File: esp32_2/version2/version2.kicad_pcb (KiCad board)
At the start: 4 copper layers, 31 x 38.5 mm, 29 parts, among them J1 USB_C_Receptacle_USB2.0_16P, J2 Conn_01x08_Pin, J3 Conn_01x08_Pin, SW1 SW_Push, SW2 SW_Push, U1 USBLC6-2SC6, U2 AP2112K-3.3, U3 ESP32-C3-WROOM-02, Y1 Crystal

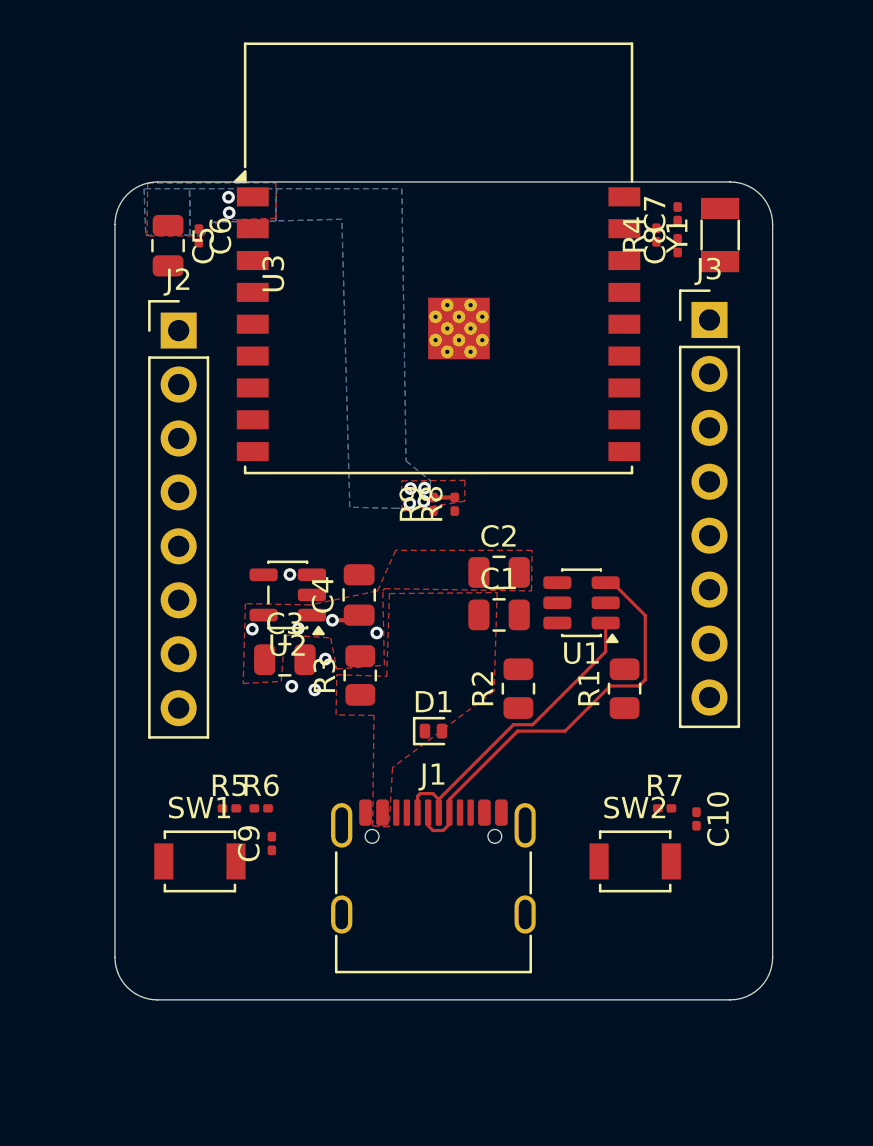
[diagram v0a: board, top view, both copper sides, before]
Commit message: fixed up some other basic routing issues i hate this
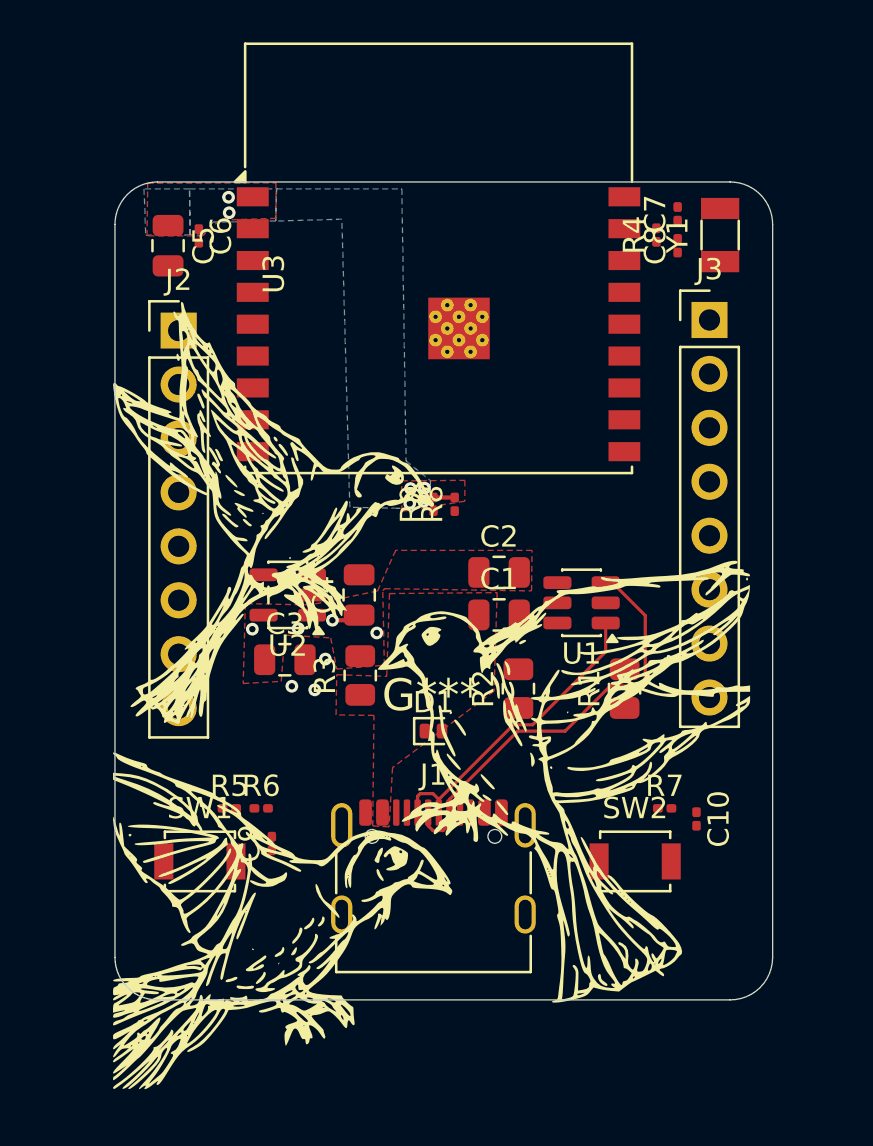
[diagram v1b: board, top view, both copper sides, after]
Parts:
- added G***: LOGO, LOGO, F.Cu at (87.4, 73.2)

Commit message: more routing more vias more visas (not)
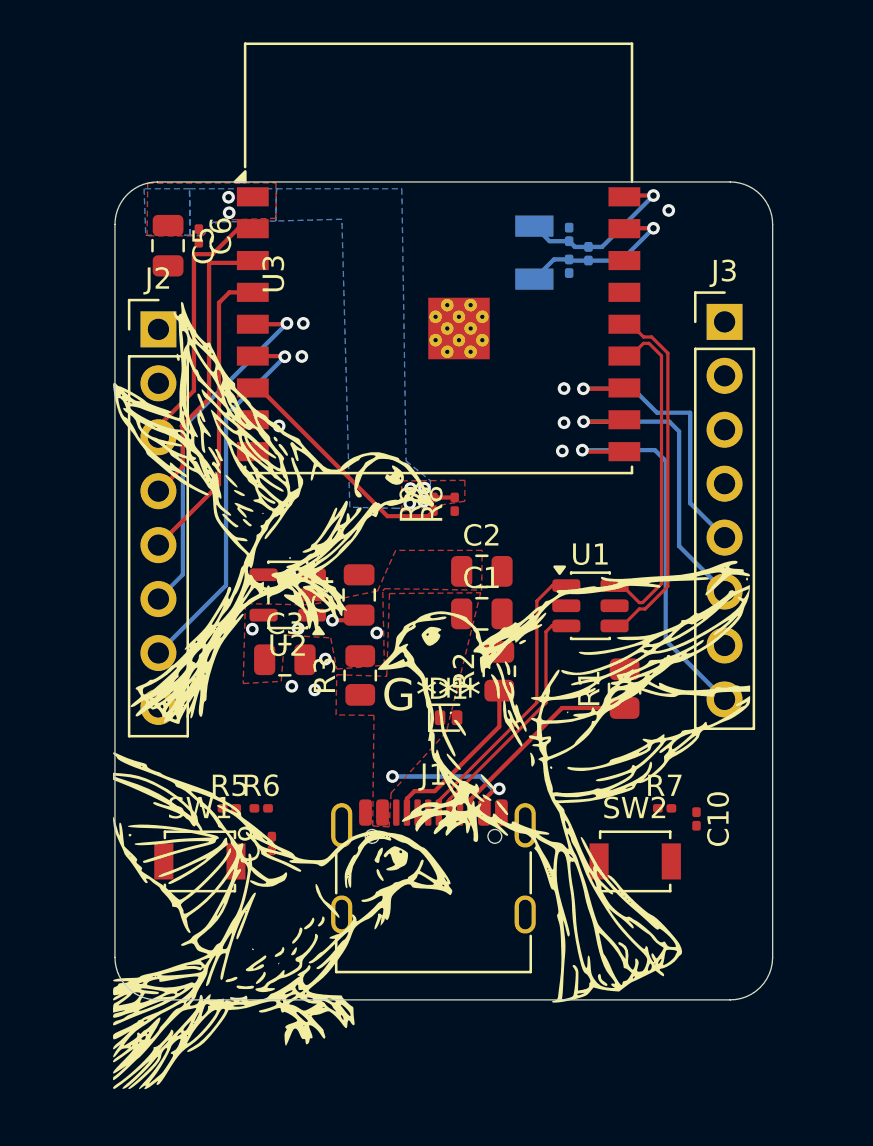
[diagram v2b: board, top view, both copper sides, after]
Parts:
- C7, C8, R4, Y1: moved to B.Cu
- moved Y1 8.79 mm to (92.2, 52.3)
- moved C7 5.20 mm to (93.9, 51.5)
- moved C8 5.20 mm to (93.9, 53.0), turned to -90 degrees
- moved R4 3.32 mm to (94.8, 52.4), turned to -90 degrees
- moved R2 1.22 mm to (90.6, 72.0)
- moved J2 0.96 mm to (74.5, 55.9)
- moved D1 0.95 mm to (88.2, 74.2)
- moved C1 0.81 mm to (89.8, 69.3)
- moved C2 0.81 mm to (89.8, 67.3)
- moved J3 0.72 mm to (101.2, 55.6)
- moved U1 0.44 mm to (94.9, 69.0), turned to 0 degrees
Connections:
- U3 pad 11: IO13 -> RXD
- U3 pad 12: IO14 -> TXD
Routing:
- net IO10: track 0.00 -> 18.5 mm, vias 0 -> 1
- net IO7: track 0.00 -> 17.9 mm, vias 0 -> 1
- net IO6: track 0.00 -> 17.4 mm, vias 0 -> 1
- net USB_D+: track 0.00 -> 16.9 mm
- net USB_D-: track 0.00 -> 16.2 mm
- net RXD: track 0.00 -> 15.1 mm, vias 0 -> 1
- net IO5: track 0.00 -> 14.4 mm
- net TXD: track 0.00 -> 14.0 mm, vias 0 -> 1
- net IO4: track 0.00 -> 13.9 mm
- net EN: track 0.00 -> 12.6 mm
- net IO8: track 0.00 -> 11.1 mm
- net Net-(J1-CC2): track 0.00 -> 9.65 mm
- net Net-(U3-IO0): track 0.00 -> 8.42 mm, vias 0 -> 1
- net Net-(J1-CC1): track 0.00 -> 8.10 mm
- net /D+: track 20.1 -> 12.0 mm
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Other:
- board text added: "add in GND (IO9 = GND) near the vias because if something changes and the pcb needs to find ground, the current will spread throughout the entire pcb and can cause serious damage. better to have a GND pin right there in case something happens"

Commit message: finished routing
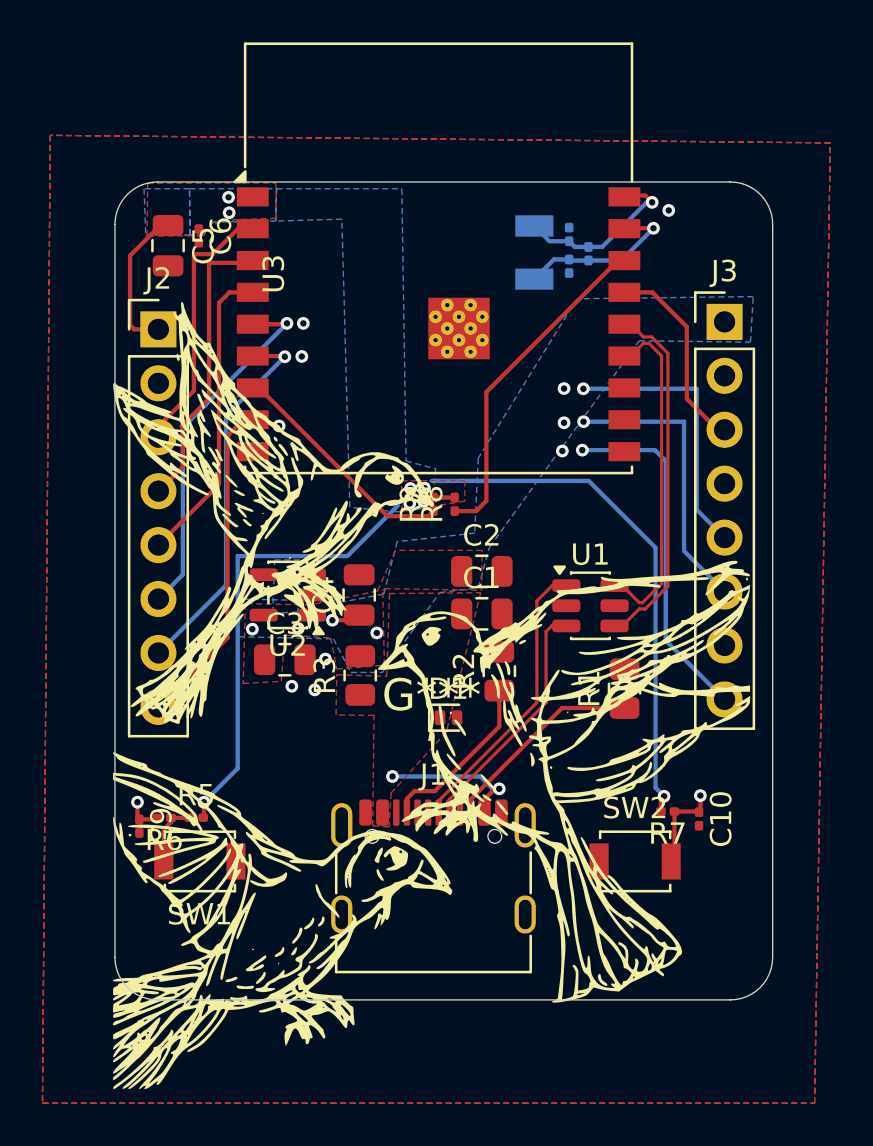
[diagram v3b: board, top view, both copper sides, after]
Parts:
- moved C9 6.29 mm to (73.7, 79.3), turned to -90 degrees
- moved R6 4.59 mm to (74.8, 79.0), turned to 180 degrees
- moved R5 1.62 mm to (76.3, 78.9)
- moved R7 0.21 mm to (98.5, 78.7), turned to 180 degrees
- moved C10 0.12 mm to (100.0, 79.0)
- turned SW1 to 180 degrees
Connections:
- C1 pad 2: IO9 -> GND
- C10 pad 2: IO9 -> GND
- C2 pad 2: IO9 -> GND
- C3 pad 2: IO9 -> GND
- C4 pad 2: IO9 -> GND
- C5 pad 2: IO9 -> GND
- C6 pad 2: IO9 -> GND
- C7 pad 2: IO9 -> GND
- C8 pad 2: IO9 -> GND
- C9 pad 2: IO9 -> GND
- D1 pad 2: IO9 -> GND
- J1 pad A1: IO9 -> GND
- J1 pad A12: IO9 -> GND
- J1 pad B1: IO9 -> GND
- J1 pad B12: IO9 -> GND
- J1 pad SH: IO9 -> GND
- J2 pad 2: IO9 -> GND
- J3 pad 2: IO9 -> GND
- J3 pad 4: IO9 -> GND
- J3 pad 7: IO9 -> GND
- R1 pad 2: IO9 -> GND
- R2 pad 2: IO9 -> GND
- R5 pad 1: IO9 -> Net-(R5-Pad1)
- R6 pad 1: IO9 -> Net-(R5-Pad1)
- SW1 pad 1: IO9 -> GND
- SW1 pad 2: IO9 -> Net-(R5-Pad1)
- SW2 pad 1: IO9 -> GND
- U1 pad 2: IO9 -> GND
- U2 pad 2: IO9 -> GND
- U3 pad 11: RXD -> IO13
- U3 pad 12: TXD -> IO14
- U3 pad 19: IO9 -> GND
- U3 pad 9: IO9 -> GND
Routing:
- net +3V3: track 1.00 -> 54.1 mm, vias 6 -> 8
- net IO9: track 0.00 -> 47.3 mm, vias 10 -> 1
- net EN: track 12.6 -> 32.5 mm, vias 0 -> 1
- net IO2: track 0.00 -> 15.9 mm
- net IO3: track 0.00 -> 9.39 mm
- net Net-(R5-Pad1): track 0.00 -> 3.06 mm
- net IO10: track 18.5 -> 16.6 mm
- net RXD: track 15.1 -> 13.5 mm
- net TXD: track 14.0 -> 12.9 mm
- net GND: vias 0 -> 10
- added copper zone on B.Cu, net +5V
- added copper zone on B.Cu, net GND
- added copper zone on F.Cu, net GND
- added copper zone on In1.Cu, net GND
- added copper zone on In2.Cu, net GND
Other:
- board text added: "add in GND near the vias because if something changes and the pcb needs to find ground, the current will spread throughout the entire pcb and can cause serious damage. better to have a GND pin right there in case something happens"
- board text removed: "add in GND (IO9 = GND) near the vias because if something changes and the pcb needs to find ground, the current will spread throughout the entire pcb and can cause serious damage. better to have a GND pin right there in case something happens"
